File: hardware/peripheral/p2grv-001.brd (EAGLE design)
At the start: 18 x 31 mm, 5 parts

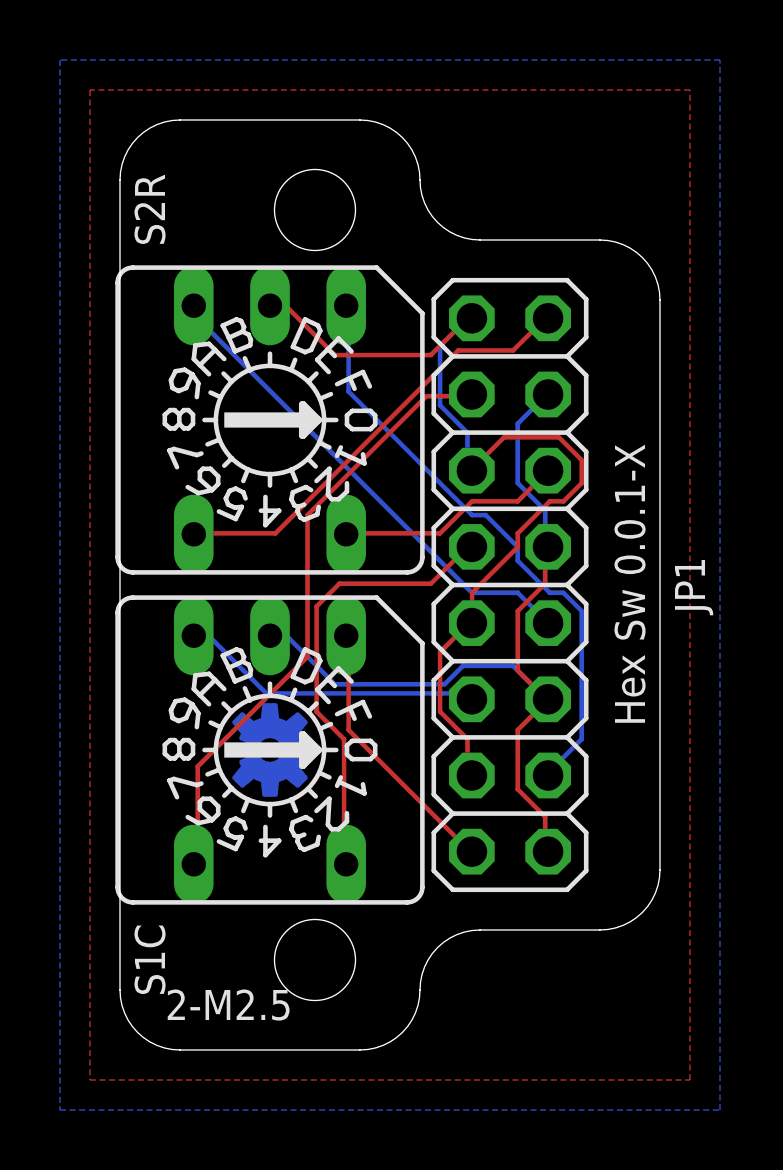
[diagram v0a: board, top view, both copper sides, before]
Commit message: WIP.
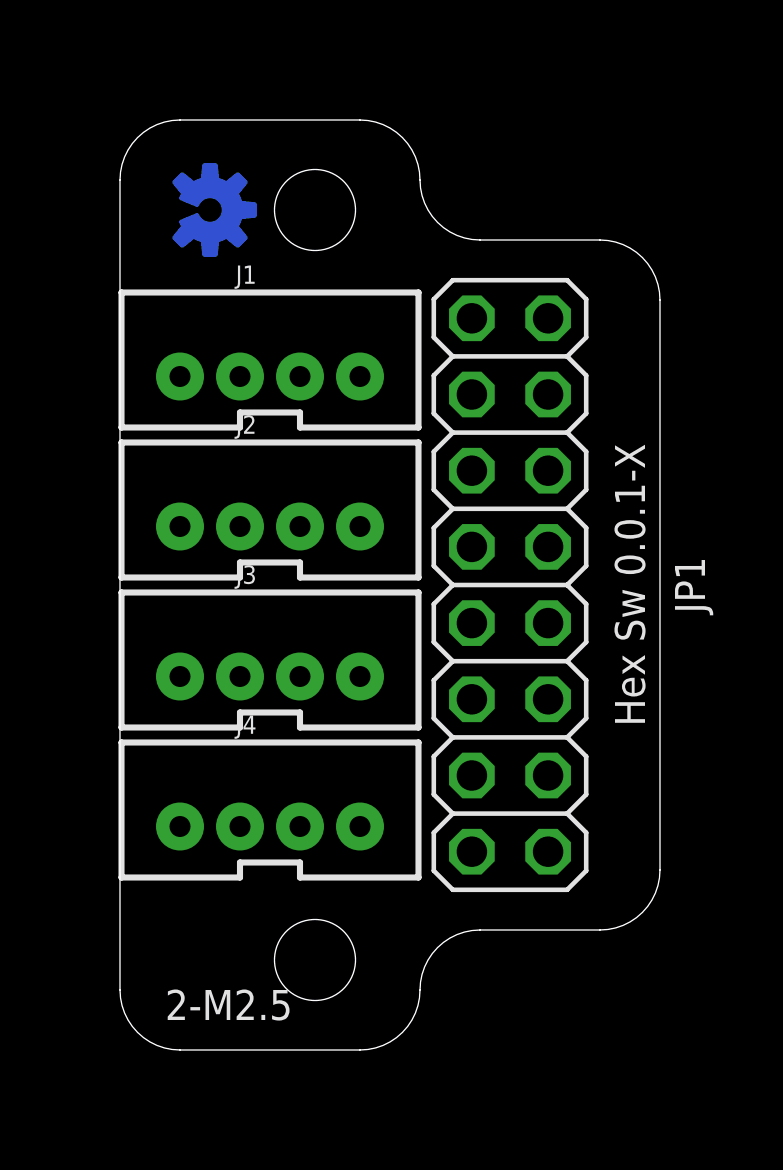
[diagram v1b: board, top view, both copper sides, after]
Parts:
- removed S1C, S2R: (no value), switch-dil:A1353HEX
- added J1, J2, J3, J4: (no value), SparkFun-Connectors:JST-4-PTH-VERT
- moved LOGO1 18.1 mm to (3.00, 28.0)
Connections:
- net ANLG0: no longer S2R.1
- net ANLG1: no longer S2R.4
- net ANLG2: no longer S2R.8
- net ANLG3: no longer S2R.2
- net DTCT0: no longer S1C.1
- net DTCT1: no longer S1C.4
- net DTCT2: no longer S1C.8
- net DTCT3: no longer S1C.2
- net GND: no longer S1C.C
- net VCC: no longer S2R.C
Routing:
- net VCC: track 31.7 -> 0.00 mm
- net GND: track 28.5 -> 0.00 mm
- net DTCT3: track 20.4 -> 0.00 mm
- net ANLG0: track 19.9 -> 0.00 mm
- net ANLG1: track 16.4 -> 0.00 mm
- net DTCT2: track 15.0 -> 0.00 mm
- net ANLG3: track 14.8 -> 0.00 mm
- net DTCT1: track 10.1 -> 0.00 mm
- net DTCT0: track 8.95 -> 0.00 mm
- net ANLG2: track 7.60 -> 0.00 mm
- removed copper zone on layer 1, net GND
- removed copper zone on layer 16, net GND
